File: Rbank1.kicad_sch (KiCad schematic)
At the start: 100 parts, among them K1 TQ2-5, K2 TQ2-5, K3 TQ2-5, K4 TQ2-5, K5 TQ2-5, K6 TQ2-5, K7 TQ2-5, K8 TQ2-5, K9 TQ2-5, Q1 2N2222, Q2 2N2222, Q3 2N2222, Q4 2N2222, Q5 2N2222, Q6 2N2222, Q7 2N2222, Q8 2N2222, Q9 2N2222

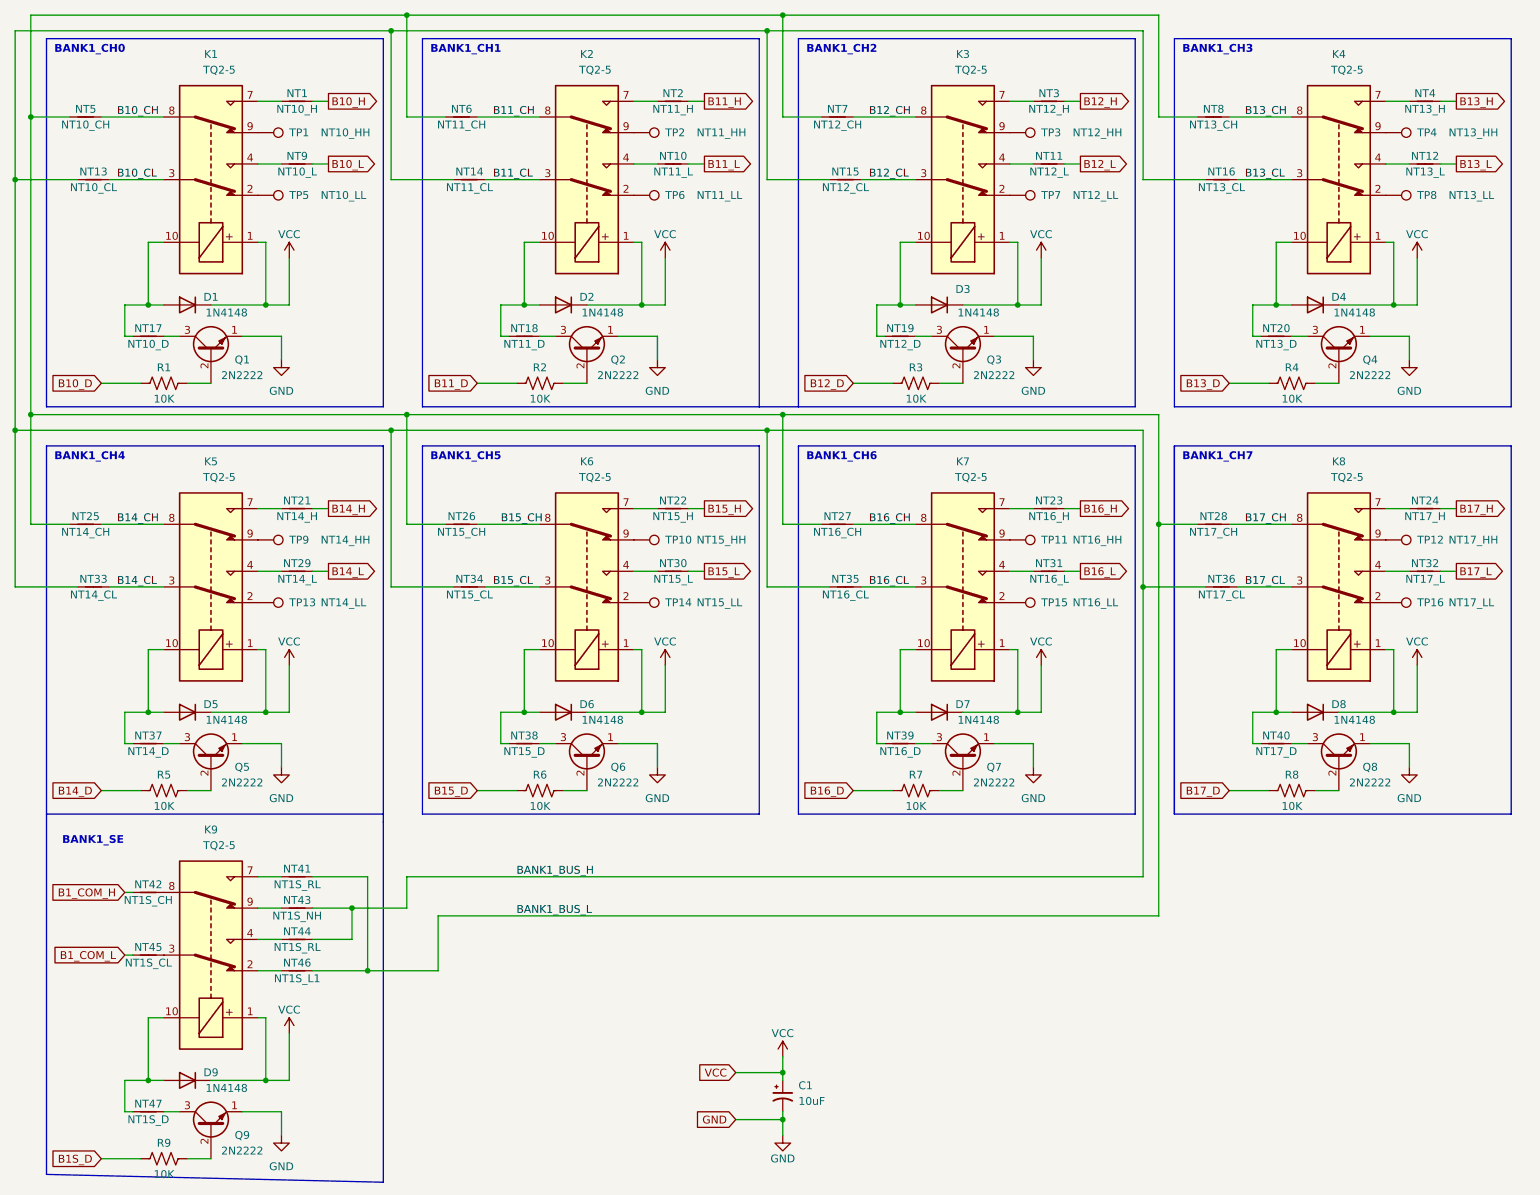
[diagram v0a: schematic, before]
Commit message: backup 1 bank done
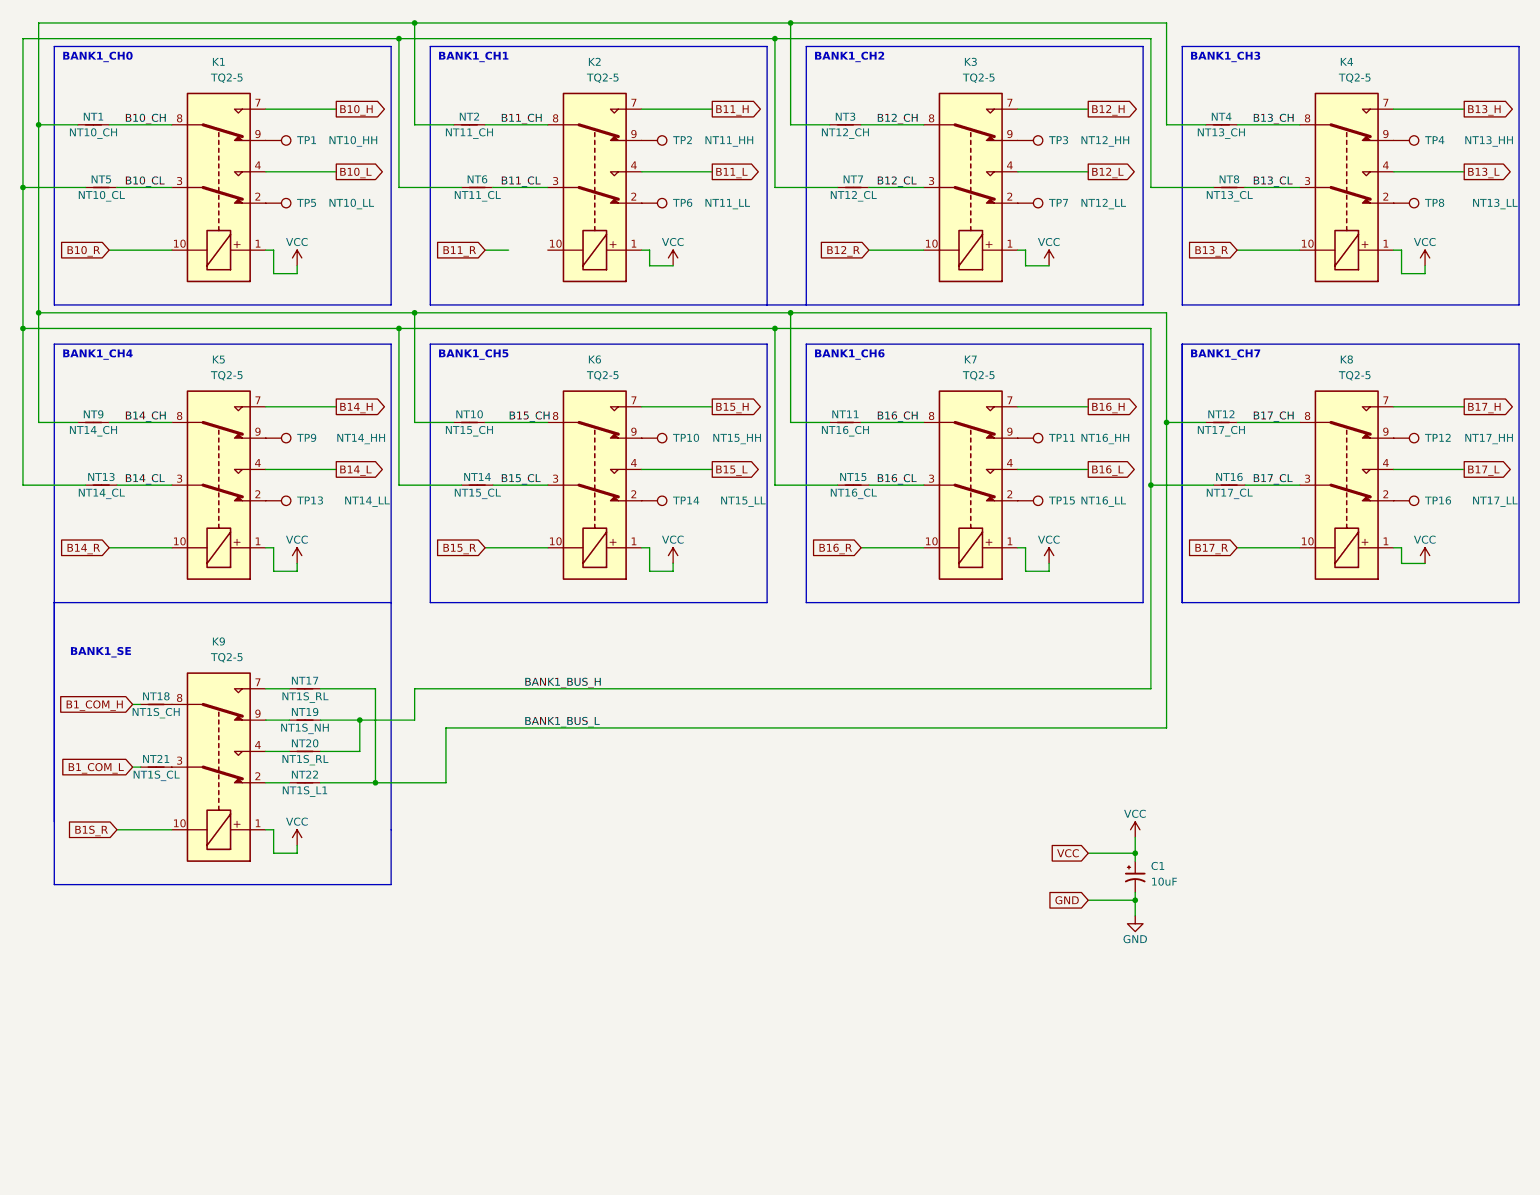
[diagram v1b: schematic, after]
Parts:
- removed D1, D2, D3, D4, D5, D6, D7, D8, D9: 1N4148, Diode_THT:D_DO-35_SOD27_P7.62mm_Horizontal, symbol Diode:1N4148
- removed NT23: NT16_H, NetTie:NetTie-2_THT_Pad1.0mm, symbol Device:NetTie_2
- removed NT24: NT17_H, NetTie:NetTie-2_THT_Pad1.0mm, symbol Device:NetTie_2
- removed NT25: NT14_CH, NetTie:NetTie-2_THT_Pad1.0mm, symbol Device:NetTie_2
- removed NT26: NT15_CH, NetTie:NetTie-2_THT_Pad1.0mm, symbol Device:NetTie_2
- removed NT27: NT16_CH, NetTie:NetTie-2_THT_Pad1.0mm, symbol Device:NetTie_2
- removed NT28: NT17_CH, NetTie:NetTie-2_THT_Pad1.0mm, symbol Device:NetTie_2
- removed NT29: NT14_L, NetTie:NetTie-2_THT_Pad1.0mm, symbol Device:NetTie_2
- removed NT30: NT15_L, NetTie:NetTie-2_THT_Pad1.0mm, symbol Device:NetTie_2
- removed NT31: NT16_L, NetTie:NetTie-2_THT_Pad1.0mm, symbol Device:NetTie_2
- removed NT32: NT17_L, NetTie:NetTie-2_THT_Pad1.0mm, symbol Device:NetTie_2
- removed NT33: NT14_CL, NetTie:NetTie-2_THT_Pad1.0mm, symbol Device:NetTie_2
- removed NT34: NT15_CL, NetTie:NetTie-2_THT_Pad1.0mm, symbol Device:NetTie_2
- removed NT35: NT16_CL, NetTie:NetTie-2_THT_Pad1.0mm, symbol Device:NetTie_2
- removed NT36: NT17_CL, NetTie:NetTie-2_THT_Pad1.0mm, symbol Device:NetTie_2
- removed NT37: NT14_D, NetTie:NetTie-2_THT_Pad1.0mm, symbol Device:NetTie_2
- removed NT38: NT15_D, NetTie:NetTie-2_THT_Pad1.0mm, symbol Device:NetTie_2
- removed NT39: NT16_D, NetTie:NetTie-2_THT_Pad1.0mm, symbol Device:NetTie_2
- removed NT40: NT17_D, NetTie:NetTie-2_THT_Pad1.0mm, symbol Device:NetTie_2
- removed NT41, NT44: NT1S_RL, NetTie:NetTie-2_THT_Pad1.0mm, symbol Device:NetTie_2
- removed NT42: NT1S_CH, NetTie:NetTie-2_THT_Pad1.0mm, symbol Device:NetTie_2
- removed NT43: NT1S_NH, NetTie:NetTie-2_THT_Pad1.0mm, symbol Device:NetTie_2
- removed NT45: NT1S_CL, NetTie:NetTie-2_THT_Pad1.0mm, symbol Device:NetTie_2
- removed NT46: NT1S_L1, NetTie:NetTie-2_THT_Pad1.0mm, symbol Device:NetTie_2
- removed NT47: NT1S_D, NetTie:NetTie-2_THT_Pad1.0mm, symbol Device:NetTie_2
- removed Q1, Q2, Q3, Q4, Q5, Q6, Q7, Q8, Q9: 2N2222, Package_TO_SOT_THT:TO-92_Inline, symbol Transistor_BJT:2N3904
- removed R1, R2, R3, R4, R5, R6, R7, R8, R9: 10K, Resistor_THT:R_Axial_DIN0309_L9.0mm_D3.2mm_P12.70mm_Horizontal, symbol Device:R_US
- NT1: value NT10_H -> NT10_CH; footprint NetTie:NetTie-2_THT_Pad1.0mm -> NetTie:NetTie-2_Front1.0mm
- NT10: value NT11_L -> NT15_CH; footprint NetTie:NetTie-2_THT_Pad1.0mm -> NetTie:NetTie-2_Front1.0mm
- NT11: value NT12_L -> NT16_CH; footprint NetTie:NetTie-2_THT_Pad1.0mm -> NetTie:NetTie-2_Front1.0mm
- NT12: value NT13_L -> NT17_CH; footprint NetTie:NetTie-2_THT_Pad1.0mm -> NetTie:NetTie-2_Front1.0mm
- NT13: value NT10_CL -> NT14_CL; footprint NetTie:NetTie-2_THT_Pad1.0mm -> NetTie:NetTie-2_Front1.0mm
- NT14: value NT11_CL -> NT15_CL; footprint NetTie:NetTie-2_THT_Pad1.0mm -> NetTie:NetTie-2_Front1.0mm
- NT15: value NT12_CL -> NT16_CL; footprint NetTie:NetTie-2_THT_Pad1.0mm -> NetTie:NetTie-2_Front1.0mm
- NT16: value NT13_CL -> NT17_CL; footprint NetTie:NetTie-2_THT_Pad1.0mm -> NetTie:NetTie-2_Front1.0mm
- NT17: value NT10_D -> NT1S_RL; footprint NetTie:NetTie-2_THT_Pad1.0mm -> NetTie:NetTie-2_Front1.0mm
- NT18: value NT11_D -> NT1S_CH; footprint NetTie:NetTie-2_THT_Pad1.0mm -> NetTie:NetTie-2_Front1.0mm
- NT19: value NT12_D -> NT1S_NH; footprint NetTie:NetTie-2_THT_Pad1.0mm -> NetTie:NetTie-2_Front1.0mm
- NT2: value NT11_H -> NT11_CH; footprint NetTie:NetTie-2_THT_Pad1.0mm -> NetTie:NetTie-2_Front1.0mm
- NT20: value NT13_D -> NT1S_RL; footprint NetTie:NetTie-2_THT_Pad1.0mm -> NetTie:NetTie-2_Front1.0mm
- NT21: value NT14_H -> NT1S_CL; footprint NetTie:NetTie-2_THT_Pad1.0mm -> NetTie:NetTie-2_Front1.0mm
- NT22: value NT15_H -> NT1S_L1; footprint NetTie:NetTie-2_THT_Pad1.0mm -> NetTie:NetTie-2_Front1.0mm
- NT3: value NT12_H -> NT12_CH; footprint NetTie:NetTie-2_THT_Pad1.0mm -> NetTie:NetTie-2_Front1.0mm
- NT4: value NT13_H -> NT13_CH; footprint NetTie:NetTie-2_THT_Pad1.0mm -> NetTie:NetTie-2_Front1.0mm
- NT5: value NT10_CH -> NT10_CL; footprint NetTie:NetTie-2_THT_Pad1.0mm -> NetTie:NetTie-2_Front1.0mm
- NT6: value NT11_CH -> NT11_CL; footprint NetTie:NetTie-2_THT_Pad1.0mm -> NetTie:NetTie-2_Front1.0mm
- NT7: value NT12_CH -> NT12_CL; footprint NetTie:NetTie-2_THT_Pad1.0mm -> NetTie:NetTie-2_Front1.0mm
- NT8: value NT13_CH -> NT13_CL; footprint NetTie:NetTie-2_THT_Pad1.0mm -> NetTie:NetTie-2_Front1.0mm
- NT9: value NT10_L -> NT14_CH; footprint NetTie:NetTie-2_THT_Pad1.0mm -> NetTie:NetTie-2_Front1.0mm
- TP1, TP10, TP11, TP12, TP13, TP14, TP15, TP16, TP2, TP3, TP4, TP5, TP6, TP7, TP8, TP9: footprint Connector_Pin:Pin_D1.0mm_L10.0mm -> Connector_Pin:Pin_D0.9mm_L10.0mm_W2.4mm_FlatFork
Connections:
- net B10_CH: now also NT1.2; no longer NT5.2
- net B10_CL: now also NT5.2; no longer NT13.2
- net B10_H: now also K1.7; no longer NT1.2
- net B10_L: now also K1.4; no longer NT9.2
- net B11_CH: now also NT2.2; no longer NT6.2
- net B11_CL: now also NT6.2; no longer NT14.2
- net B11_H: now also K2.7; no longer NT2.2
- net B11_L: now also K2.4; no longer NT10.2
- net B12_CH: now also NT3.2; no longer NT7.2
- net B12_CL: now also NT7.2; no longer NT15.2
- net B12_H: now also K3.7; no longer NT3.2
- net B12_L: now also K3.4; no longer NT11.2
- net B13_CH: now also NT4.2; no longer NT8.2
- net B13_CL: now also NT8.2; no longer NT16.2
- net B13_H: now also K4.7; no longer NT4.2
- net B13_L: now also K4.4; no longer NT12.2
- net B14_CH: now also NT9.2
- net B14_CL: now also NT13.2
- net B14_H: now also K5.7; no longer NT21.2
- net B14_L: now also K5.4
- net B15_CH: now also NT10.2
- net B15_CL: now also NT14.2
- net B15_H: now also K6.7; no longer NT22.2
- net B15_L: now also K6.4
- net B16_CH: now also NT11.2
- net B16_CL: now also NT15.2
- net B16_H: now also K7.7
- net B16_L: now also K7.4
- net B17_CH: now also NT12.2
- net B17_CL: now also NT16.2
- net B17_H: now also K8.7
- net B17_L: now also K8.4
- net B1_COM_H: now also NT18.1
- net B1_COM_L: now also NT21.1
- net BANK1_BUS_H: now also NT19.2, NT20.2, NT5.1, NT6.1, NT7.1, NT8.1
- net BANK1_BUS_L: now also NT1.1, NT10.1, NT11.1, NT12.1, NT17.2, NT2.1, NT22.2, NT3.1, NT4.1, NT9.1; no longer NT5.1, NT6.1, NT7.1, NT8.1
- net B16_R: now reaches K7.10
- net B17_R: now reaches K8.10
- net B15_R: now reaches K6.10
- net at NT22.1: now also K9.2; no longer K6.7
- net at K9.9: now also NT19.1
- net B1S_R: now reaches K9.10
- net at K2.10: no longer NT18.1
- net at K9.4: now also NT20.1
- net B13_R: now reaches K4.10
- net B13_R: no longer NT20.1
- net at K9.7: now also NT17.1
- net B10_R: now reaches K1.10
- net B10_R: no longer NT17.1
- net B12_R: now reaches K3.10
- net B12_R: no longer NT19.1
- net B14_R: now reaches K5.10
- net at NT18.2: now also K9.8
- net at K9.3: now also NT21.2
